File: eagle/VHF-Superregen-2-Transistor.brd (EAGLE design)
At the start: 43.2 x 22.9 mm, 25 parts, among them SW1 SL-SW-1P-2T-H, T1 2N3904, T2 2N3904

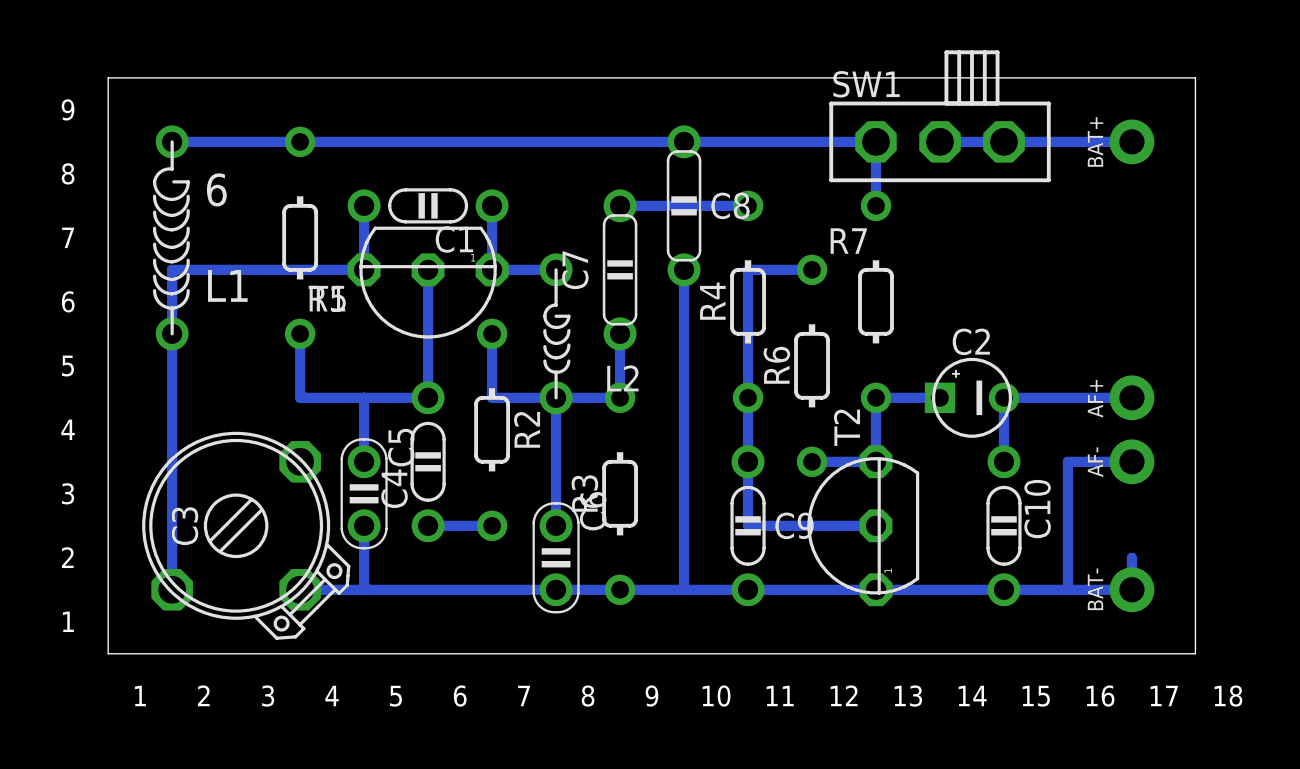
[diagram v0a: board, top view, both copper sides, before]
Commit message: ...
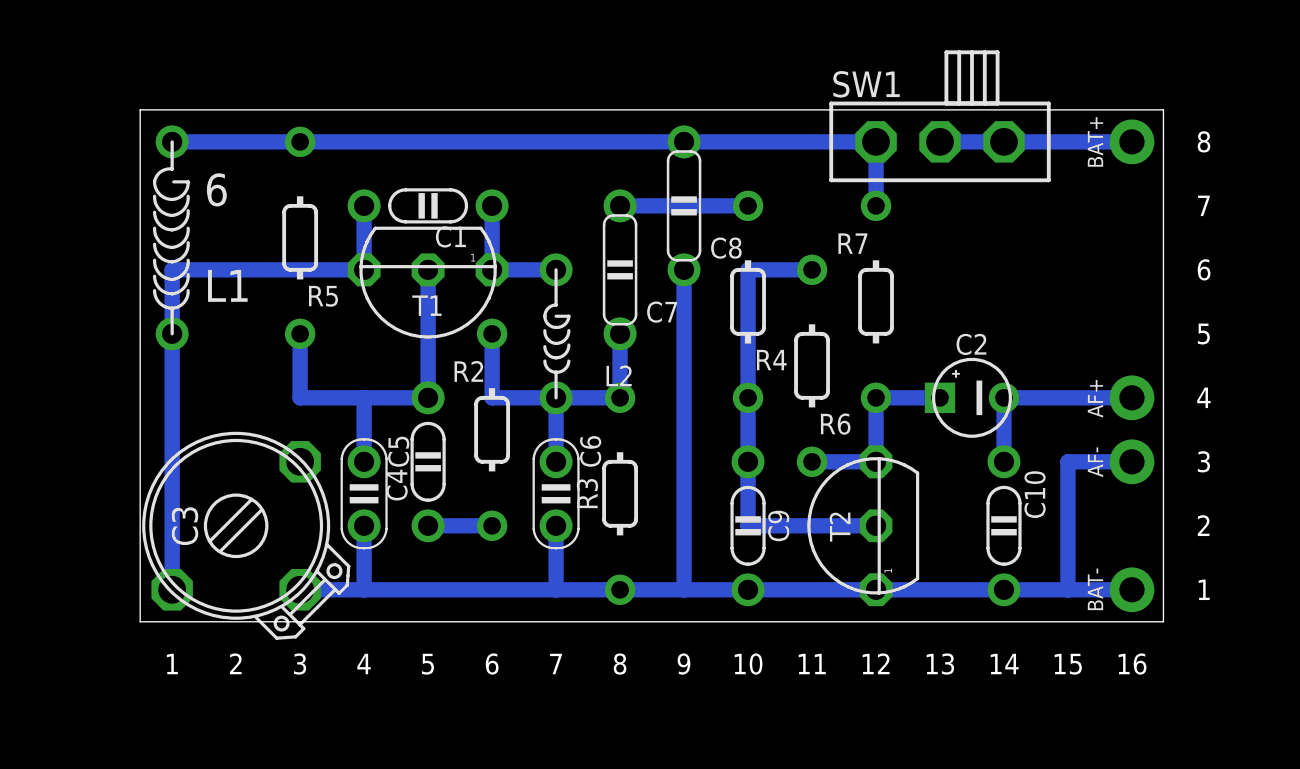
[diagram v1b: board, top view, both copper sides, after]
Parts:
- C7: device c:C050-020X044 -> c:C050-020X044/V
- L2: device r:L-02/5V -> l:L-02/5V
- R2, R4, R6: device r:0202/7 -> r:0202/7-V
- moved C6 2.54 mm to (17.8, 7.62)
- turned C7 to 180 degrees
- turned R2 to 0 degrees
- turned R4 to 180 degrees
- turned R6 to 180 degrees
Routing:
- net N$6: track 15.2 -> 12.7 mm
- net GND: track 57.1 -> 58.4 mm
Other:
- board size 43.2 x 22.9 mm -> 40.6 x 20.3 mm
- board text removed: "17"
- board text removed: "18"

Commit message: ...
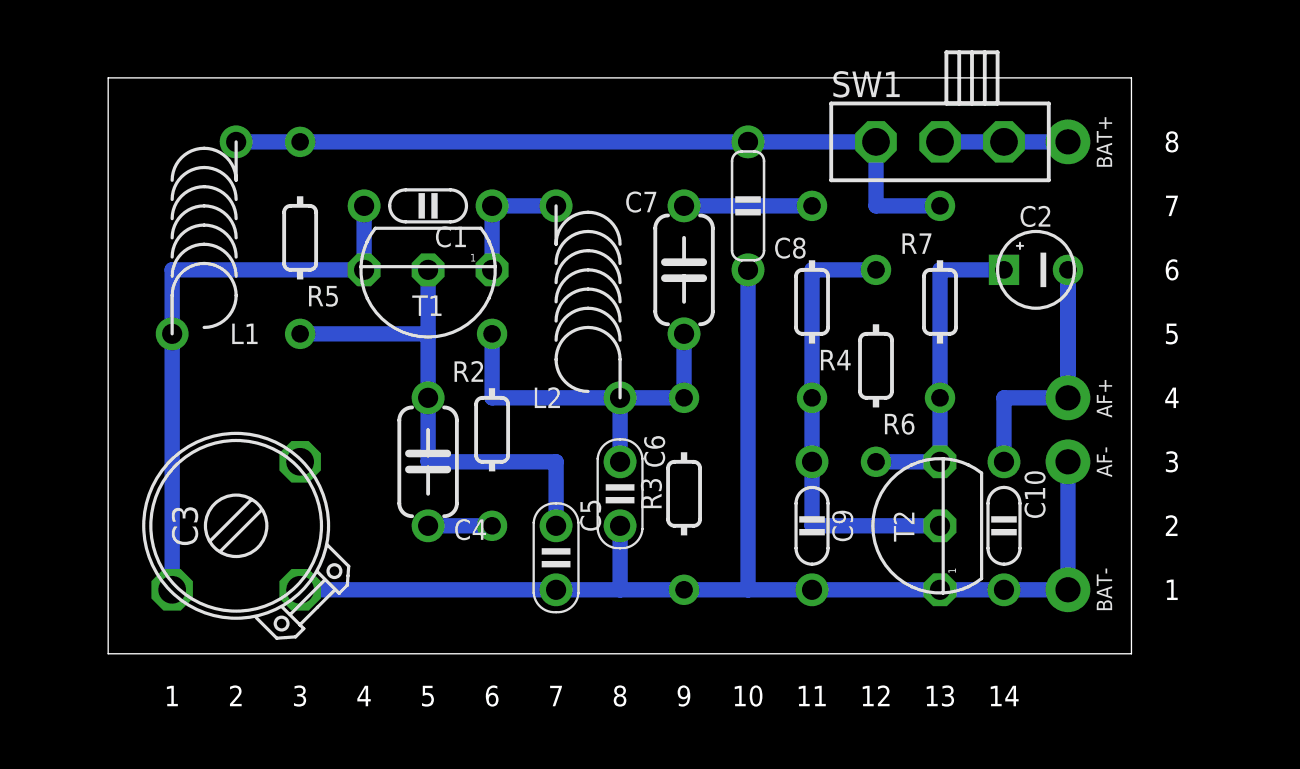
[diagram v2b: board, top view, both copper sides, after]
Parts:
- C4: device c:C050-020X036 -> c:C050-024X044/V
- C7: device c:C050-020X044/V -> c:C050-024X044/V
- L1: device r:L-02/7V -> l:L-04/7V-X
- L2: device l:L-02/5V -> l:L-04/7V
- moved C5 8.03 mm to (17.8, 5.08)
- moved C2 5.68 mm to (36.8, 15.2)
- moved L2 2.84 mm to (19.1, 15.2), turned to 0 degrees
- moved C9 2.54 mm to (27.9, 5.08)
- moved R4 2.54 mm to (27.9, 14.0)
- moved R7 2.54 mm to (33.0, 14.0)
- moved T2 2.54 mm to (33.0, 5.08)
- moved AF+ 2.54 mm to (38.1, 10.2), turned to 180 degrees
- moved AF- 2.54 mm to (38.1, 7.62), turned to 180 degrees
- moved BAT+ 2.54 mm to (38.1, 20.3), turned to 180 degrees
- moved BAT- 2.54 mm to (38.1, 2.54), turned to 180 degrees
- moved C6 2.54 mm to (20.3, 7.62)
- moved C7 2.54 mm to (22.9, 15.2), turned to 0 degrees
- moved C8 2.54 mm to (25.4, 17.8)
- moved R3 2.54 mm to (22.9, 6.35)
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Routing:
- net N$11: track 7.62 -> 15.2 mm
- net GND: track 58.4 -> 50.8 mm
- net N$4: track 15.2 -> 20.3 mm
- net N$5: track 7.62 -> 12.7 mm
- net N$9: track 7.62 -> 5.08 mm
- net N$6: track 12.7 -> 15.2 mm
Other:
- board size 40.6 x 20.3 mm -> 40.6 x 22.9 mm
- board text removed: "15"
- board text removed: "16"
